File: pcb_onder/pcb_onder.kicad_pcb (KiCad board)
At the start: 2 copper layers, 15 parts, among them J1 Conn_01x10_Female

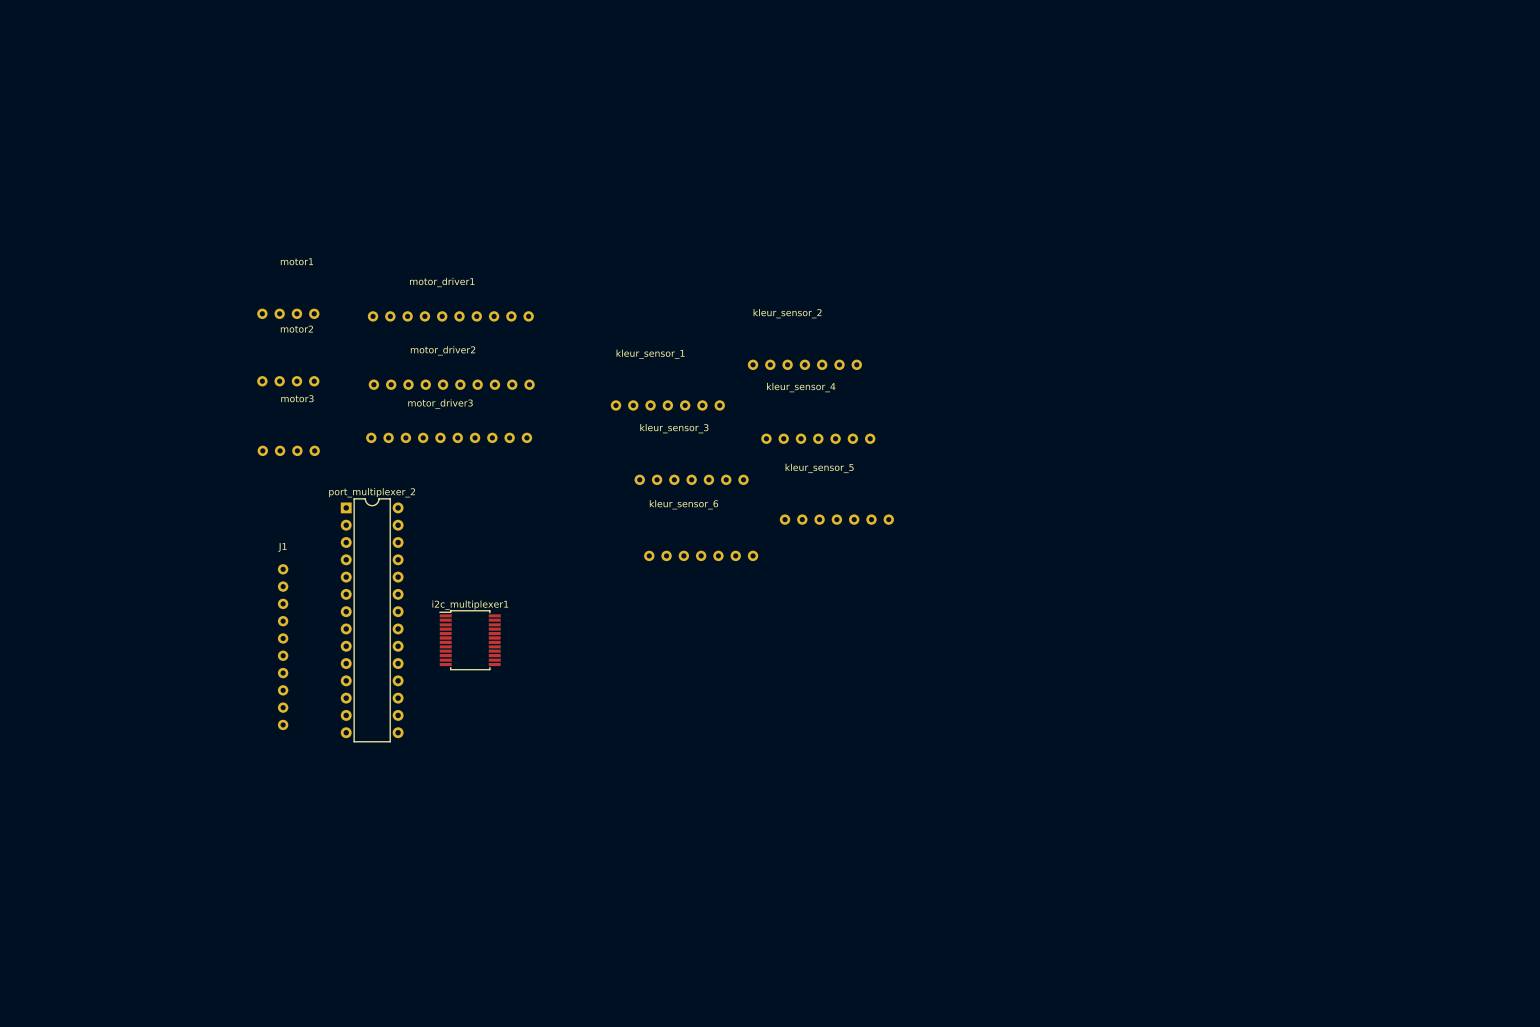
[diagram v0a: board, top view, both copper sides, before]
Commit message: lower_pcb
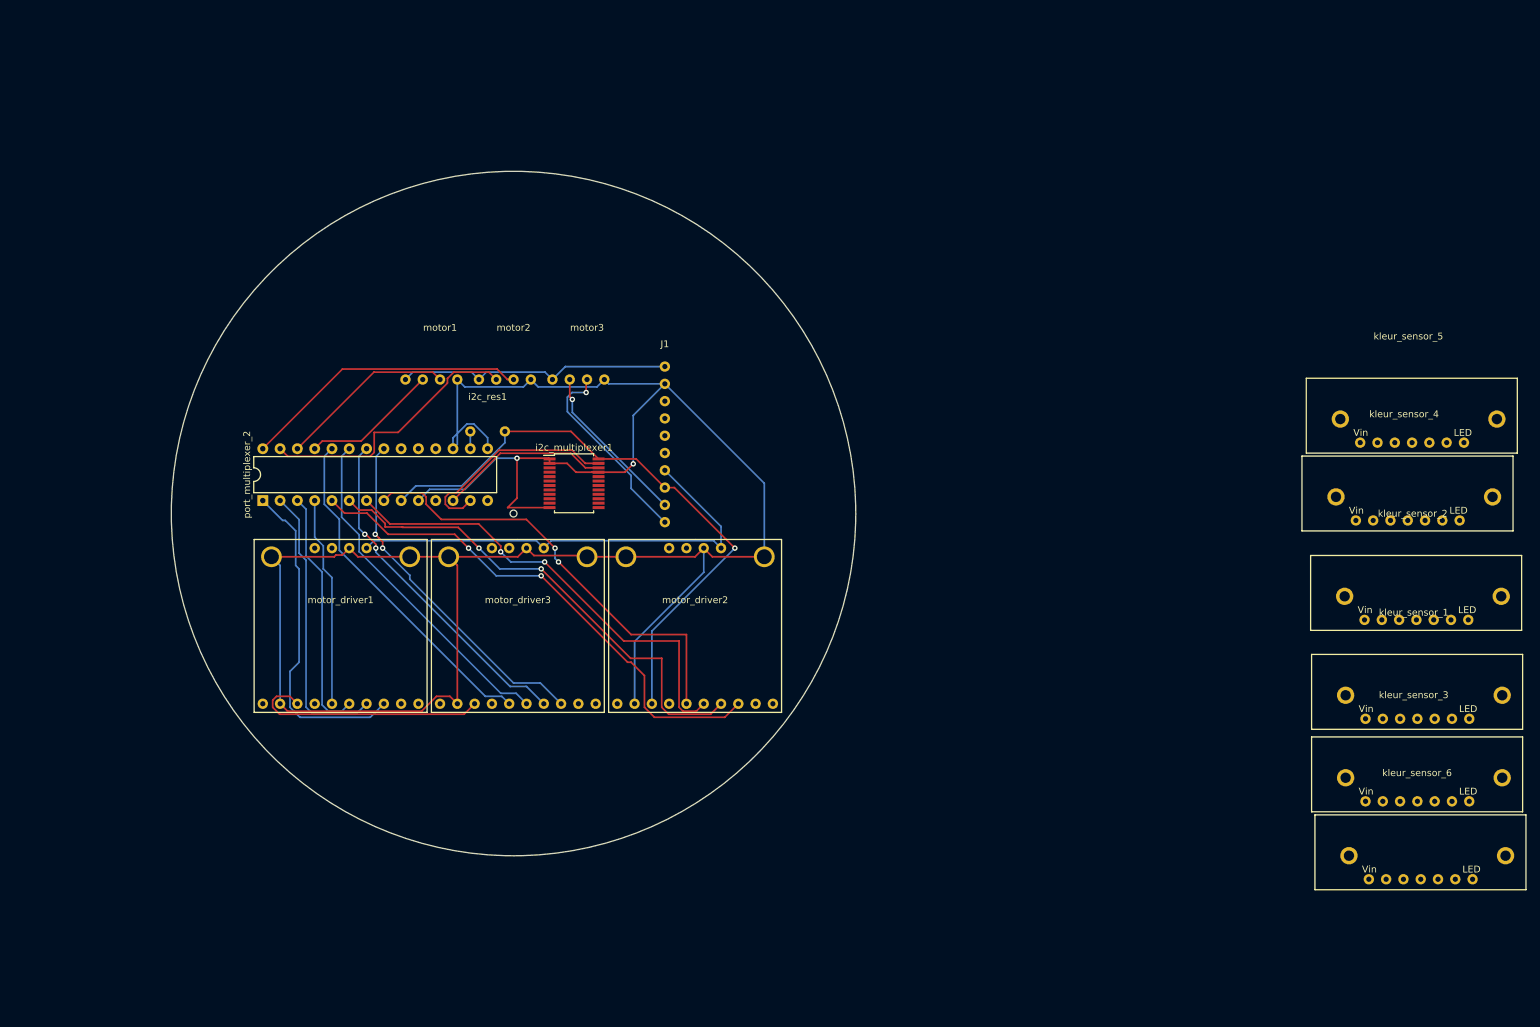
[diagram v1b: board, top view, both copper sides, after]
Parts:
- added i2c_res1: R, custom:resistor, F.Cu at (110.5, 89.5)
- moved kleur_sensor_1 118.4 mm to (246.5, 126.3)
- moved kleur_sensor_3 115.5 mm to (246.5, 138.4)
- moved kleur_sensor_6 114.7 mm to (247.0, 149.9)
- moved kleur_sensor_2 96.4 mm to (246.4, 111.8)
- moved kleur_sensor_4 88.7 mm to (245.1, 97.2)
- moved kleur_sensor_5 88.6 mm to (245.7, 85.7)
- moved J1 63.5 mm to (136.5, 82.5)
- moved motor_driver2 52.1 mm to (141.0, 119.4)
- moved motor_driver1 49.1 mm to (88.9, 119.4)
- moved motor3 43.8 mm to (125.1, 81.9)
- moved motor2 31.8 mm to (114.3, 81.9)
- moved motor_driver3 31.0 mm to (114.9, 119.4)
- moved i2c_multiplexer1 27.6 mm to (123.2, 97.2)
- moved motor1 23.1 mm to (103.5, 81.9)
- moved port_multiplexer_2 12.3 mm to (77.5, 99.7), turned to 90 degrees
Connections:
- J1 pad 5: sd6 -> Net-(J1-Pad5)
- J1 pad 6: sc6 -> Net-(J1-Pad6)
- i2c_multiplexer1 pad 1: Net-(i2c_multiplexer1-Pad1) -> gnd
- i2c_multiplexer1 pad 17: sd6 -> Net-(i2c_multiplexer1-Pad17)
- i2c_multiplexer1 pad 18: sc6 -> Net-(i2c_multiplexer1-Pad18)
- i2c_multiplexer1 pad 2: Net-(i2c_multiplexer1-Pad2) -> gnd
- i2c_multiplexer1 pad 21: Net-(i2c_multiplexer1-Pad21) -> gnd
- kleur_sensor_1 pad 5: (no net) -> Net-(kleur_sensor_1-Pad5)
- kleur_sensor_1 pad 6: (no net) -> Net-(kleur_sensor_1-Pad6)
- kleur_sensor_1 pad 7: (no net) -> Net-(kleur_sensor_1-Pad7)
- kleur_sensor_2 pad 5: (no net) -> Net-(kleur_sensor_2-Pad5)
- kleur_sensor_2 pad 6: (no net) -> Net-(kleur_sensor_2-Pad6)
- kleur_sensor_2 pad 7: (no net) -> gnd
- kleur_sensor_3 pad 5: (no net) -> Net-(kleur_sensor_3-Pad5)
- kleur_sensor_3 pad 6: (no net) -> Net-(kleur_sensor_3-Pad6)
- kleur_sensor_3 pad 7: (no net) -> gnd
- kleur_sensor_4 pad 5: (no net) -> Net-(kleur_sensor_4-Pad5)
- kleur_sensor_4 pad 6: (no net) -> Net-(kleur_sensor_4-Pad6)
- kleur_sensor_4 pad 7: (no net) -> gnd
- kleur_sensor_5 pad 5: (no net) -> Net-(kleur_sensor_5-Pad5)
- kleur_sensor_5 pad 6: (no net) -> Net-(kleur_sensor_5-Pad6)
- kleur_sensor_5 pad 7: (no net) -> gnd
- kleur_sensor_6 pad 5: (no net) -> Net-(kleur_sensor_6-Pad5)
- kleur_sensor_6 pad 6: (no net) -> Net-(kleur_sensor_6-Pad6)
- kleur_sensor_6 pad 7: (no net) -> gnd
- motor_driver1 pad 14: (no net) -> Net-(motor_driver1-Pad14)
- motor_driver2 pad 14: (no net) -> Net-(motor_driver2-Pad14)
- motor_driver3 pad 14: (no net) -> Net-(motor_driver3-Pad14)
- port_multiplexer_2 pad 12: Net-(port_multiplexer_2-Pad12) -> scl
- port_multiplexer_2 pad 13: Net-(port_multiplexer_2-Pad13) -> sda
- port_multiplexer_2 pad 15: Net-(port_multiplexer_2-Pad15) -> gnd
- port_multiplexer_2 pad 17: Net-(port_multiplexer_2-Pad17) -> gnd
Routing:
- net gnd: track 0.00 -> 323.6 mm, vias 0 -> 2
- net 3.3v: track 0.00 -> 125.3 mm, vias 0 -> 1
- net Net-(motor_driver2-Pad12): track 0.00 -> 76.4 mm, vias 0 -> 2
- net Net-(motor_driver2-Pad11): track 0.00 -> 72.8 mm, vias 0 -> 2
- net Net-(motor_driver2-Pad10): track 0.00 -> 69.0 mm, vias 0 -> 2
- net 12v: track 0.00 -> 68.7 mm
- net Net-(motor_driver2-Pad9): track 0.00 -> 65.2 mm, vias 0 -> 2
- net Net-(motor_driver3-Pad12): track 0.00 -> 51.6 mm, vias 0 -> 2
- net Net-(motor_driver3-Pad11): track 0.00 -> 50.7 mm, vias 0 -> 2
- net Net-(motor_driver3-Pad9): track 0.00 -> 50.6 mm
- net Net-(motor_driver3-Pad10): track 0.00 -> 50.5 mm
- net Net-(motor_driver1-Pad12): track 0.00 -> 48.6 mm
- net Net-(motor2-Pad3): track 0.00 -> 42.3 mm
- net Net-(motor_driver1-Pad11): track 0.00 -> 41.9 mm
- net 5v: track 0.00 -> 40.7 mm
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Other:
- board outline added: 100.5 x 100.5 mm

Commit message: lower pcb
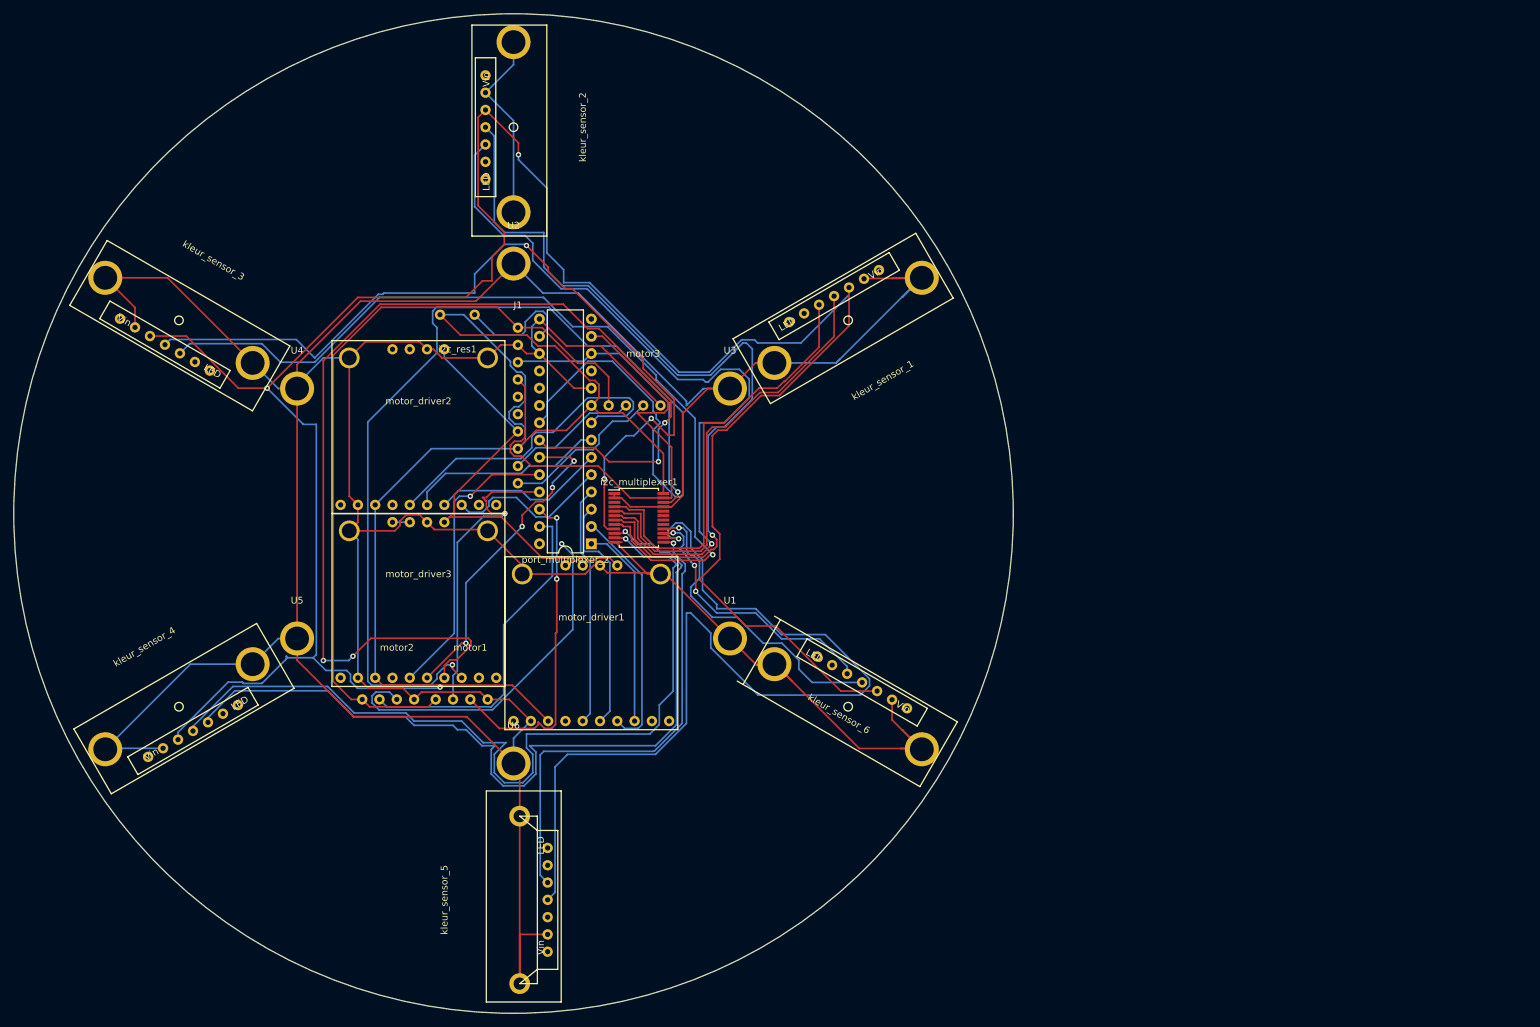
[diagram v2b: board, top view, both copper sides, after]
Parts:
- added U1: screw_hole, custom:screwhole, F.Cu at (146.1, 120.0)
- added U2: screw_hole, custom:screwhole, F.Cu at (114.3, 64.9)
- added U3: screw_hole, custom:screwhole, F.Cu at (146.1, 83.2)
- added U4: screw_hole, custom:screwhole, F.Cu at (82.5, 83.2)
- added U5: screw_hole, custom:screwhole, F.Cu at (82.5, 120.0)
- added U6: screw_hole, custom:screwhole, F.Cu at (114.3, 138.3)
- moved kleur_sensor_3 192.7 mm to (65.2, 73.2), turned to 330 degrees
- moved kleur_sensor_4 182.9 mm to (65.2, 130.0), turned to 30 degrees
- moved kleur_sensor_5 150.2 mm to (114.3, 158.3), turned to 90 degrees
- moved kleur_sensor_2 148.1 mm to (114.3, 44.9), turned to 270 degrees
- moved kleur_sensor_1 98.6 mm to (163.4, 73.2), turned to 210 degrees
- moved kleur_sensor_6 85.9 mm to (163.4, 130.0), turned to 150 degrees
- moved motor_driver2 50.0 mm to (100.3, 90.2)
- moved motor2 50.0 mm to (97.2, 128.9)
- moved port_multiplexer_2 48.7 mm to (125.7, 106.0), turned to 180 degrees
- moved motor1 47.2 mm to (108.0, 128.9)
- moved motor_driver1 36.9 mm to (125.7, 121.9)
- moved J1 22.3 mm to (114.9, 76.8)
- moved i2c_res1 17.7 mm to (106.0, 72.4), turned to 180 degrees
- moved motor_driver3 15.1 mm to (100.3, 115.6)
- moved i2c_multiplexer1 10.8 mm to (132.7, 102.2)
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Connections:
- kleur_sensor_1 pad 7: Net-(kleur_sensor_1-Pad7) -> gnd
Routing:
- net 3.3v: track 125.3 -> 523.7 mm, vias 1 -> 3
- net gnd: track 323.6 -> 708.6 mm, vias 2 -> 0
- net Net-(i2c_multiplexer1-Pad14): track 0.00 -> 141.6 mm, vias 0 -> 1
- net Net-(i2c_multiplexer1-Pad8): track 0.00 -> 128.7 mm, vias 0 -> 1
- net Net-(i2c_multiplexer1-Pad11): track 0.00 -> 126.3 mm, vias 0 -> 1
- net Net-(i2c_multiplexer1-Pad9): track 0.00 -> 126.0 mm, vias 0 -> 3
- net Net-(i2c_multiplexer1-Pad10): track 0.00 -> 123.5 mm, vias 0 -> 1
- net Net-(motor_driver3-Pad12): track 51.6 -> 172.4 mm, vias 2 -> 1
- net Net-(i2c_multiplexer1-Pad7): track 0.00 -> 119.3 mm, vias 0 -> 1
- net Net-(motor_driver3-Pad11): track 50.7 -> 163.7 mm, vias 2 -> 4
- net Net-(i2c_multiplexer1-Pad6): track 0.00 -> 112.6 mm, vias 0 -> 1
- net 5v: track 40.7 -> 116.8 mm
- net Net-(i2c_multiplexer1-Pad13): track 0.00 -> 70.9 mm, vias 0 -> 1
- net Net-(i2c_multiplexer1-Pad5): track 0.00 -> 65.4 mm
- net Net-(i2c_multiplexer1-Pad4): track 0.00 -> 63.7 mm
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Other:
- board size 100.5 x 100.5 mm -> 146.8 x 146.8 mm
